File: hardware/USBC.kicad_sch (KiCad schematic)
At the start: 16 parts, among them J601 USB_C_Receptacle_USB2.0_16P, U601 CDSOT236-0504C, U602 USBLC6-2P6, U603 CP2102N-A02-GQFN20

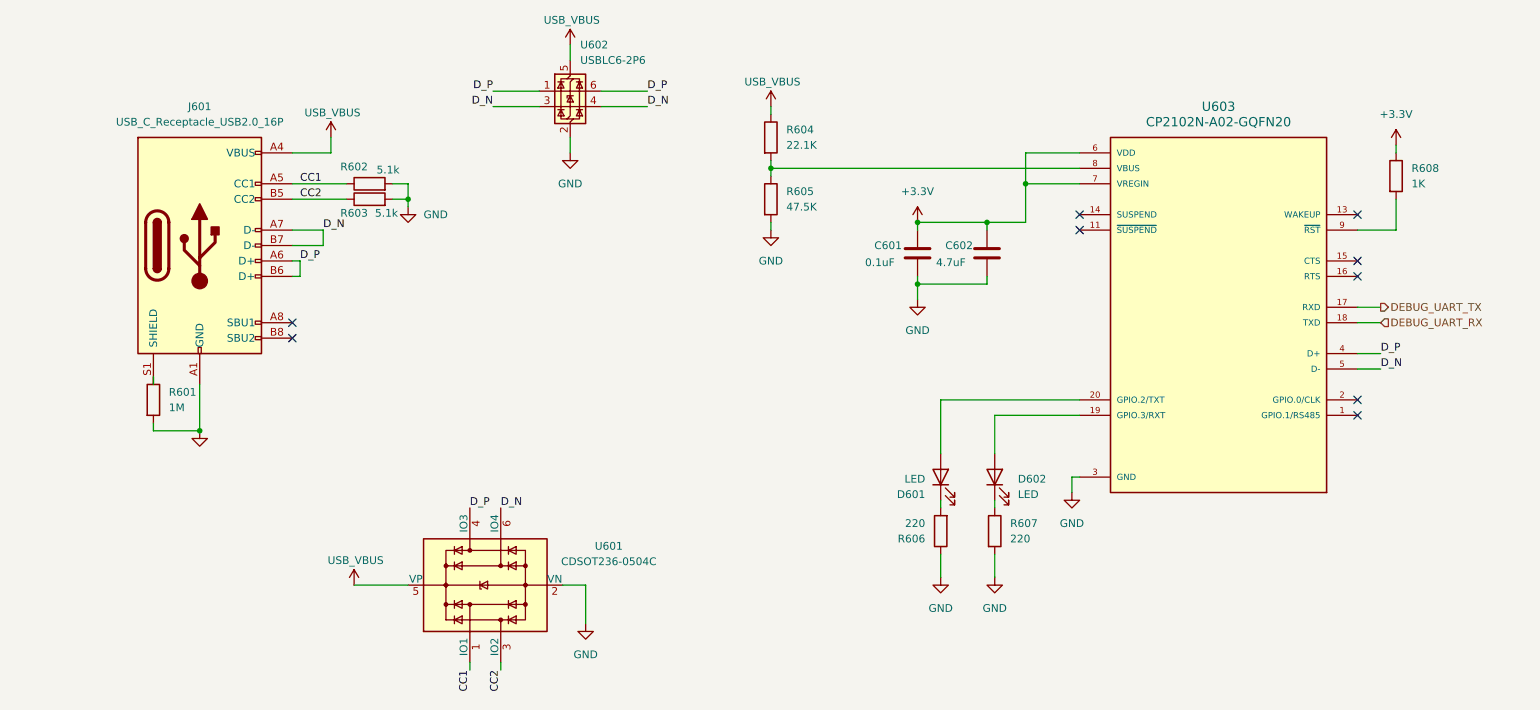
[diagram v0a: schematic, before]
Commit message: wip
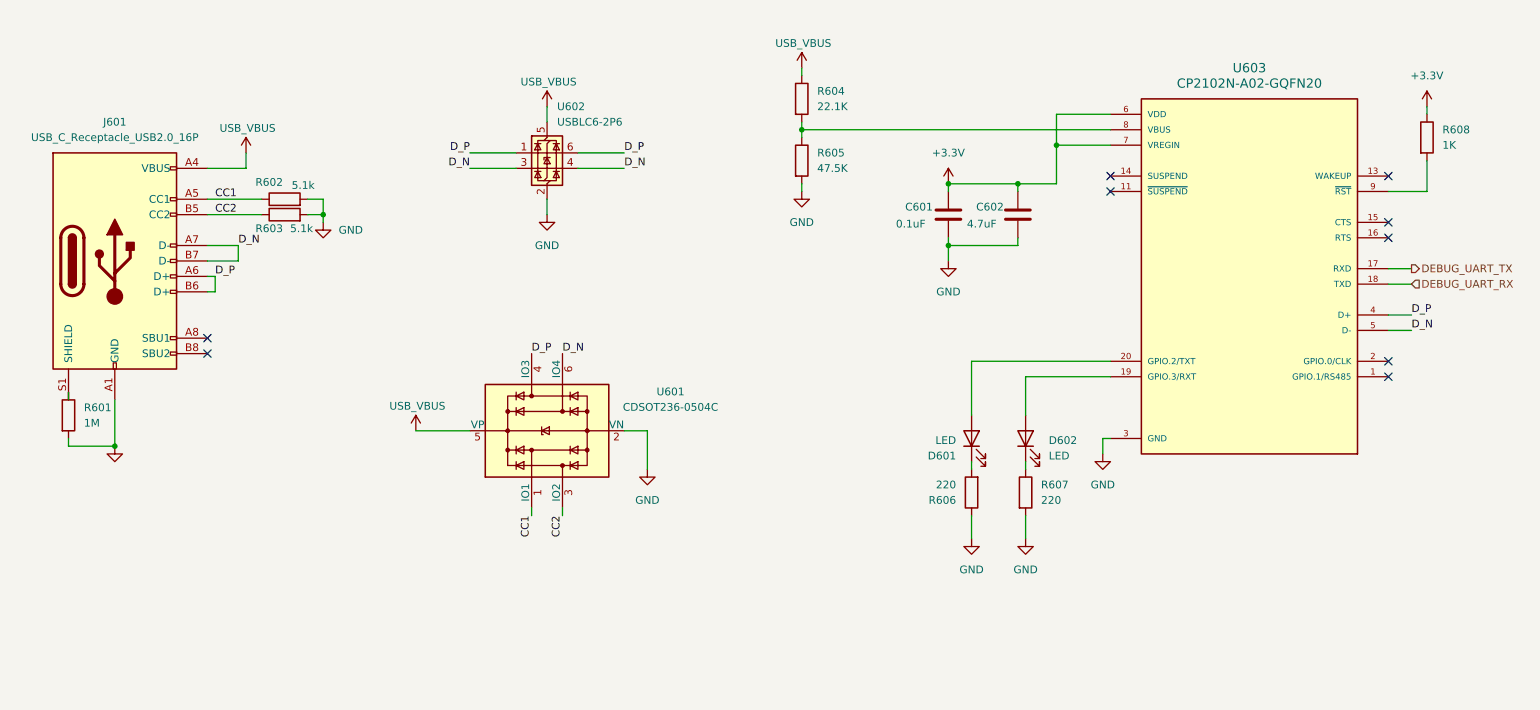
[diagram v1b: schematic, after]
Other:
- moved on the sheet: C601, C602, D601, D602, J601, R601, R602, R603, R604, R605, R606, R607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
